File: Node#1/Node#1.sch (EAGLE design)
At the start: 5 parts, among them U1 BLUENRG-232

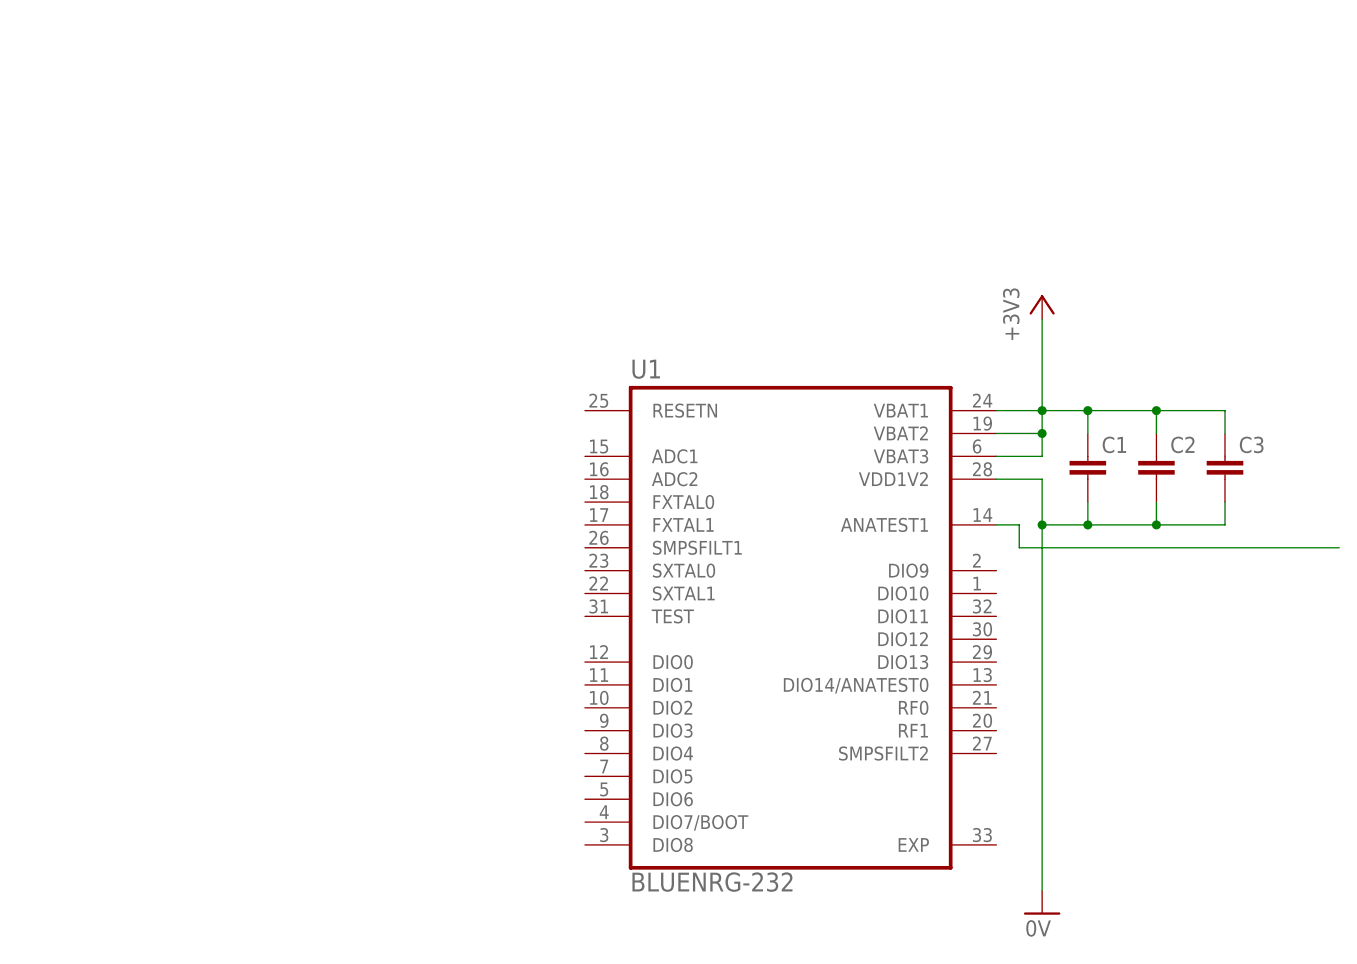
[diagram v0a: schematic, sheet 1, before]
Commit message: Modified Lib, Node#1
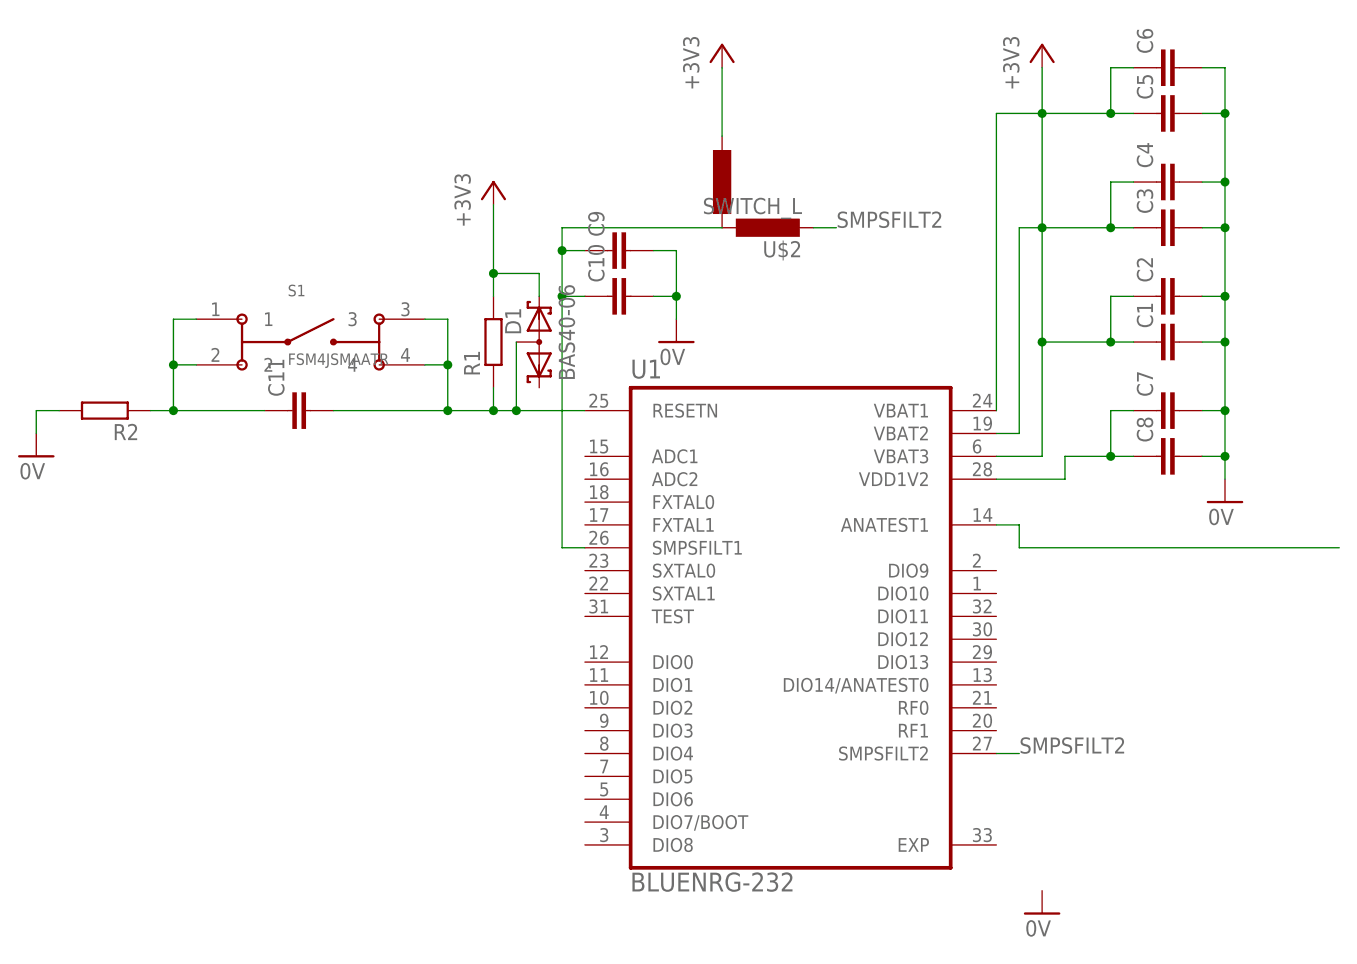
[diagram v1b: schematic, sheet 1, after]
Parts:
- added C10, C4, C5, C6, C7, C8, C9: (no value), rcl:C-EUC0805K
- added C11: (no value), rcl:C-EUC0805
- added D1: BAS40-06, diode:BAS40-06
- added R1, R2: (no value), rcl:R-EU_R0805
- added S1: FSM4JSMAATR, BlueHome:FSM4JSMAATR
- added U$2: SWITCH_L, BlueHome:SWITCH_L
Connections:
- new net N$1: C7.1, C8.1, U1.VDD1V2
- new net N$2: C10.1, C9.1, U$2.1, U1.SMPSFILT1
- new net N$3: C11.2, D1.AA, R1.1, S1.3, S1.4, U1.RESETN
- new net N$5: C11.1, R2.1, S1.1, S1.2
- new net SMPSFILT2: U$2.2, U1.SMPSFILT2
- net +3V3: now also C4.1, C5.1, C6.1, D1.K2, R1.2, U$2.3
- net 0V: now also C10.2, C4.2, C5.2, C6.2, C7.2, C8.2, C9.2, R2.2; no longer U1.VDD1V2
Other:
- moved on the sheet: C1, C2, C3
